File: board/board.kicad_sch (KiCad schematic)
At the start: 10 parts, among them J1 Screw_Terminal_01x02, J2 Screw_Terminal_01x03, J3 Screw_Terminal_01x02, J4 Screw_Terminal_01x02, U1 ADS1232IPW, U2 TPS7A20xxxDQN

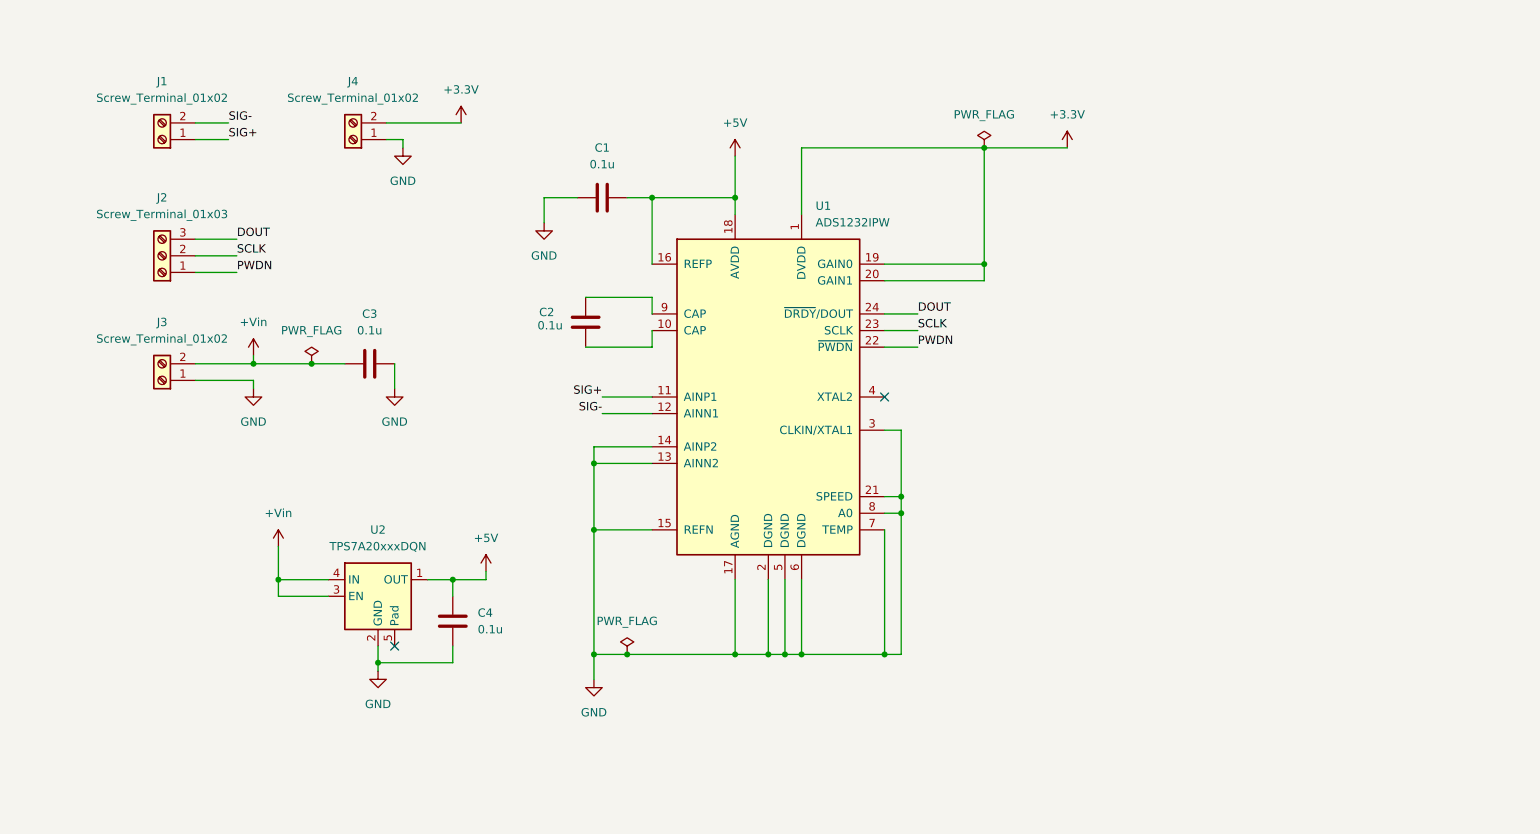
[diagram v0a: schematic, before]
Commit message: new design
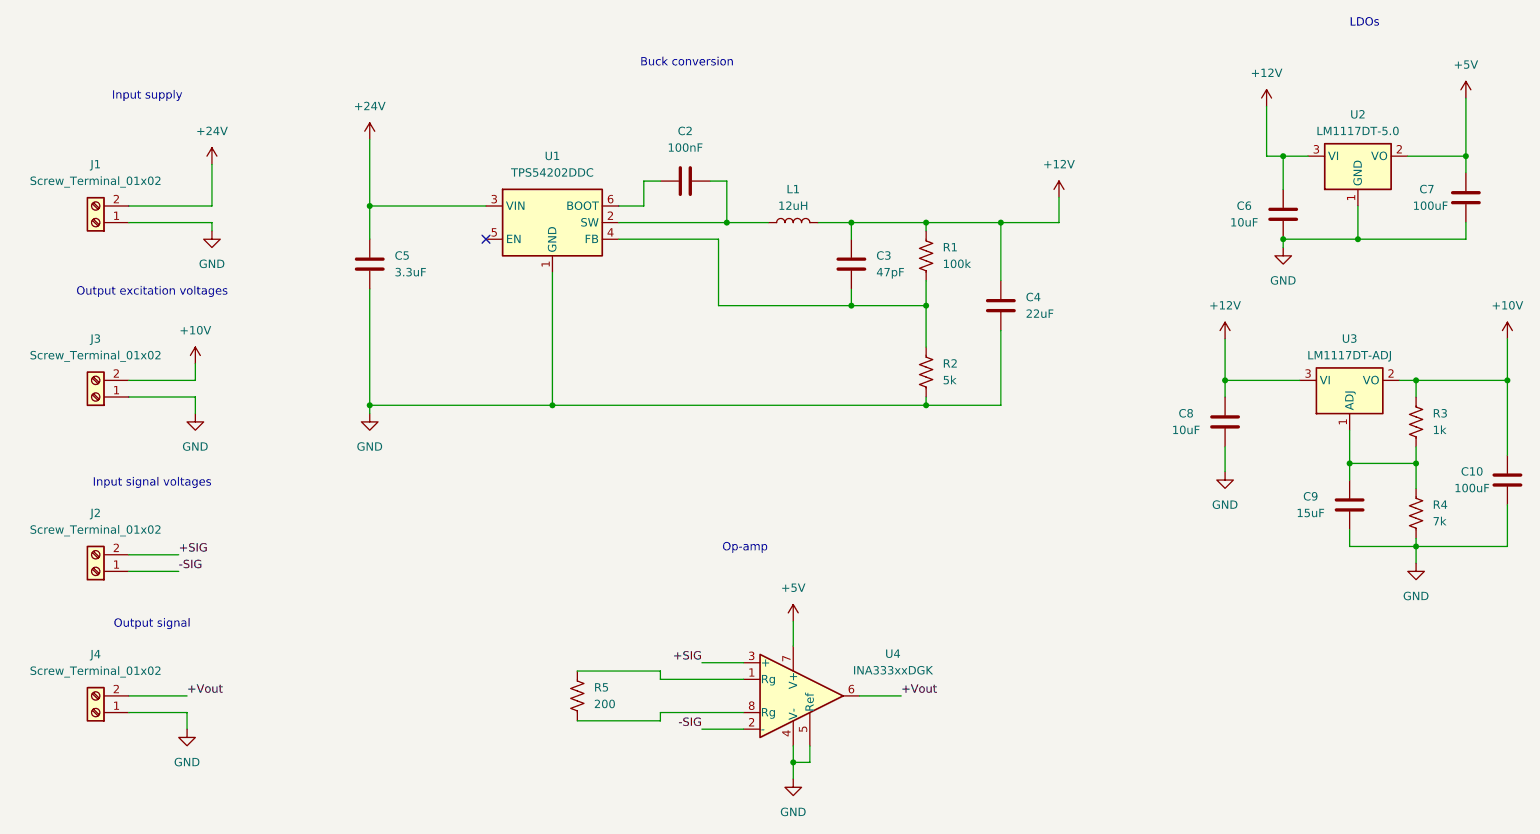
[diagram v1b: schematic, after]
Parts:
- removed C1: 0.1u, symbol Device:C
- removed J2: Screw_Terminal_01x03, symbol Connector:Screw_Terminal_01x03
- removed U1: ADS1232IPW, symbol Analog_ADC:ADS1232IPW
- removed U2: TPS7A20xxxDQN, Package_SON:Texas_X2SON-4_1x1mm_P0.65mm, symbol Regulator_Linear:TPS7A20xxxDQN
- added C10, C7: 100uF, symbol Device:C
- added C5: 3.3uF, symbol Device:C
- added C6, C8: 10uF, symbol Device:C
- added C9: 15uF, symbol Device:C
- added J2: Screw_Terminal_01x02, symbol Connector:Screw_Terminal_01x02
- added L1: 12uH, symbol Device:L
- added R1: 100k, symbol Device:R_US
- added R2: 5k, symbol Device:R_US
- added R3: 1k, symbol Device:R_US
- added R4: 7k, symbol Device:R_US
- added R5: 200, symbol Device:R_US
- added U1: TPS54202DDC, Package_TO_SOT_SMD:SOT-23-6, symbol Regulator_Switching:TPS54202DDC
- added U2: LM1117DT-5.0, Package_TO_SOT_SMD:TO-252-3_TabPin2, symbol Regulator_Linear:LM1117DT-5.0
- added U3: LM1117DT-ADJ, Package_TO_SOT_SMD:TO-252-3_TabPin2, symbol Regulator_Linear:LM1117DT-ADJ
- added U4: INA333xxDGK, Package_SO:VSSOP-8_3x3mm_P0.65mm, symbol Amplifier_Instrumentation:INA333xxDGK
- C2: value 0.1u -> 100nF
- C3: value 0.1u -> 47pF
- C4: value 0.1u -> 22uF
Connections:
- net SIG+ is gone; now on net GND: J1.1 (Pin_1)
- net +5V: now also C7.2, U2.2 (VO), U4.7 (V+); no longer C4.1
- net GND: now also C4.1, C10.1, C5.1, C6.1, C7.1, C8.1, C9.1, R2.2, R4.2, U1.1 (GND), U2.1 (GND), U4.4 (V-), U4.5 (Ref); no longer C3.1, C4.2
- net at C2.1: now also U1.6 (BOOT)
- net at C2.2: now also L1.1, U1.2 (SW)
- net +3.3V renamed +Vout
- net +Vout: now also U4.6
- net +Vin renamed +10V
- net +10V: now also C10.2, R3.1, U3.2 (VO); no longer C3.2
- net SIG- renamed +24V
- net +24V: now also C5.2, U1.3 (VIN)
- new net: C9.2, R3.2, R4.1, U3.1 (ADJ)
- new net: C3.1, R1.2, R2.1, U1.4 (FB)
- new net: R5.2, U4.1 (Rg)
- new net: R5.1, U4.8 (Rg)
- new net +12V: C3.2, C4.2, C6.2, C8.2, L1.2, R1.1, U2.3 (VI), U3.3 (VI)
- new net +SIG: J2.2 (Pin_2), U4.3 (+)
- new net -SIG: J2.1 (Pin_1), U4.2 (-)
- no-connect marks 2 -> 1
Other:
- note added: "Buck conversion"
- note added: "Input signal voltages"
- note added: "Input supply"
- note added: "LDOs"
- note added: "Op-amp"
- note added: "Output excitation voltages"
- note added: "Output signal"
